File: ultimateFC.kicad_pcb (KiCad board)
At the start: 6 copper layers, 36 x 36 mm, 213 parts, among them J1 USB_B_Micro, SW1 SW_Push, U1 LMR33630CQRNX, U2 TPS62824ADMQ, U3 LMR33620CRNXT, U4 S25FL064L, U5 DPS310, U6 BMI270, U7 STM32H735VGH6, U8 ICM-20602, Y1 CSTNE8M00G550000R0

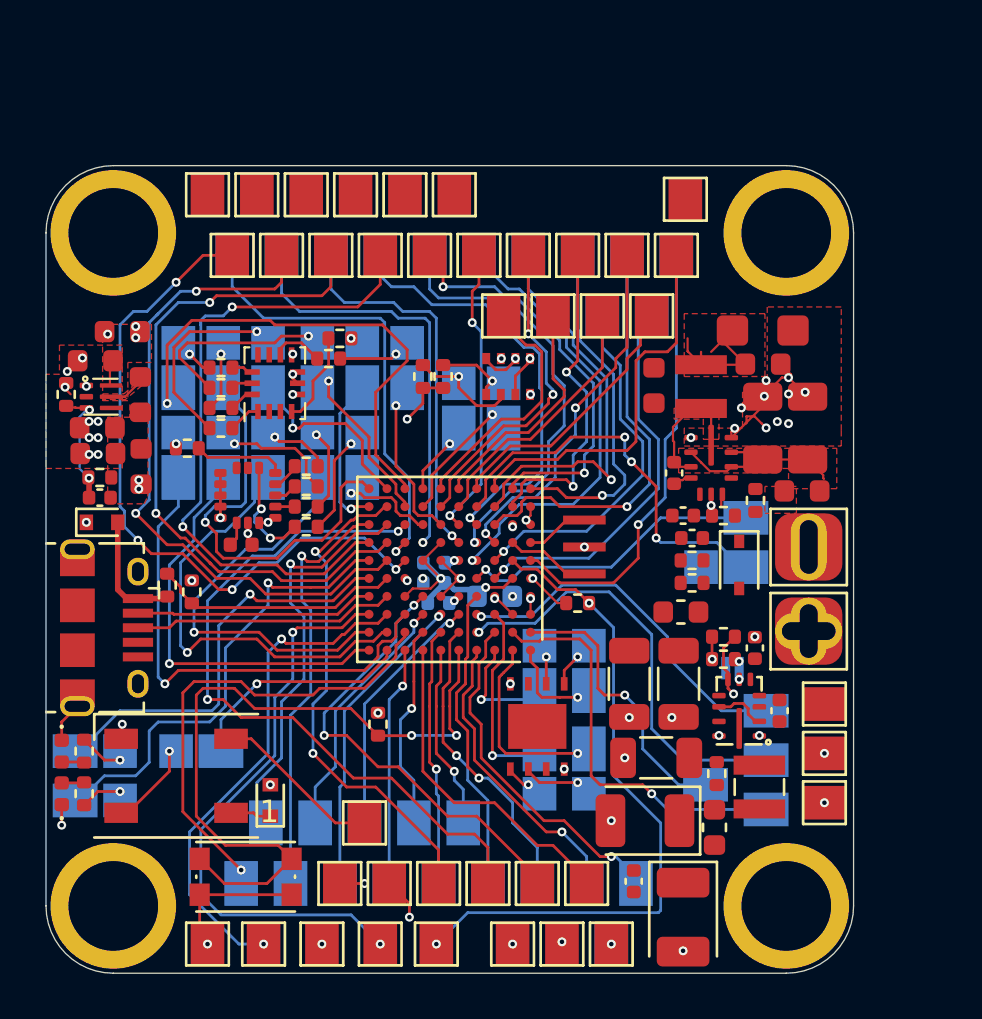
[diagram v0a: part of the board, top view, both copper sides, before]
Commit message: MORE PADS!!!
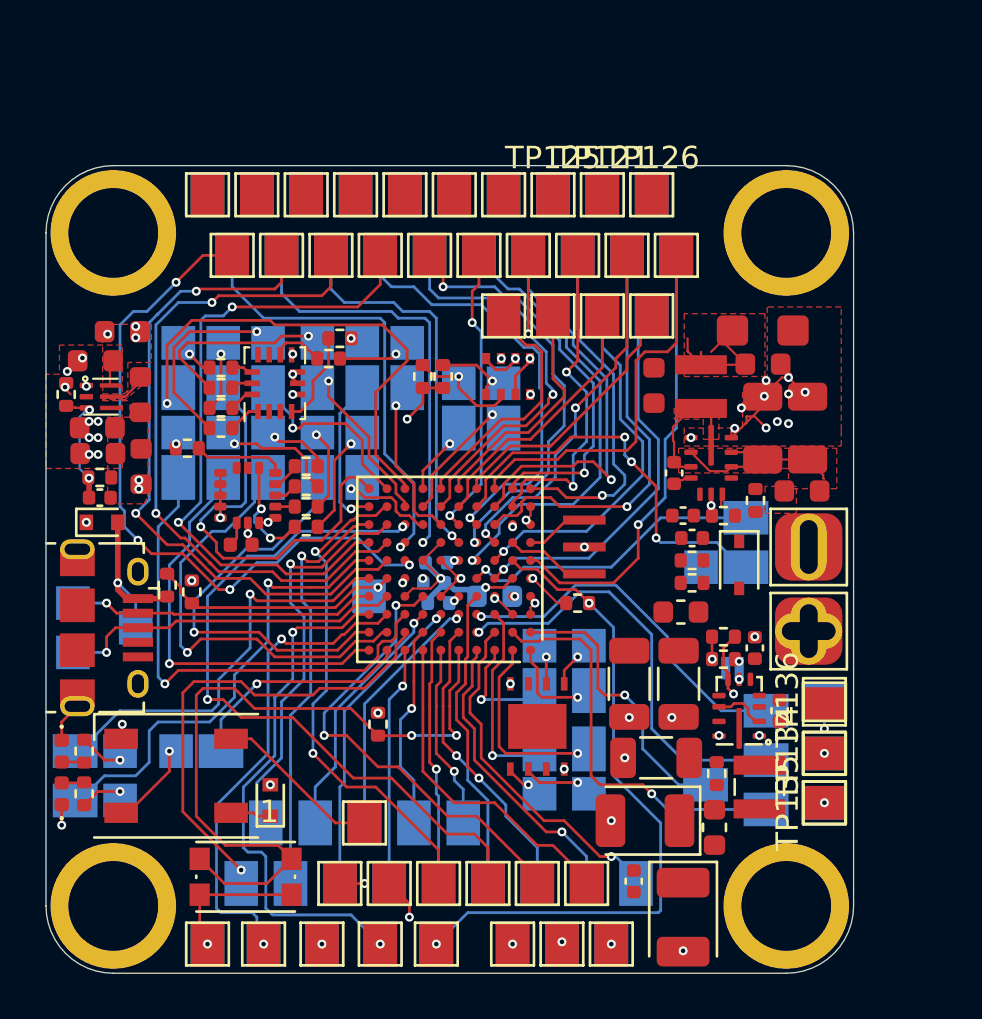
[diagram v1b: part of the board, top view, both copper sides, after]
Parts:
- added TP117: Pad, TestPoint:TestPoint_Pad_1.5x1.5mm, B.Cu at (111.4, 116.2)
- added TP118: Pad, TestPoint:TestPoint_Pad_1.5x1.5mm, B.Cu at (101.0, 117.6)
- added TP119: Pad, TestPoint:TestPoint_Pad_1.5x1.5mm, B.Cu at (98.2, 116.5)
- added TP120: Pad, TestPoint:TestPoint_Pad_1.5x1.5mm, B.Cu at (98.2, 118.7)
- added TP121: Pad, TestPoint:TestPoint_Pad_1.5x1.5mm, F.Cu at (121.8, 98.3)
- added TP122: Pad, TestPoint:TestPoint_Pad_1.5x1.5mm, B.Cu at (121.8, 98.3)
- added TP123: Pad, TestPoint:TestPoint_Pad_1.5x1.5mm, B.Cu at (108.6, 98.3)
- added TP124: Pad, TestPoint:TestPoint_Pad_1.5x1.5mm, B.Cu at (106.4, 98.3)
- added TP125: Pad, TestPoint:TestPoint_Pad_1.5x1.5mm, F.Cu at (119.6, 98.3)
- added TP126: Pad, TestPoint:TestPoint_Pad_1.5x1.5mm, F.Cu at (124.0, 98.3)
- added TP127: Pad, TestPoint:TestPoint_Pad_1.5x1.5mm, B.Cu at (110.8, 98.3)
- added TP128: Pad, TestPoint:TestPoint_Pad_1.5x1.5mm, B.Cu at (119.6, 98.3)
- added TP129: Pad, TestPoint:TestPoint_Pad_1.5x1.5mm, B.Cu at (117.4, 98.3)
- added TP130: Pad, TestPoint:TestPoint_Pad_1.5x1.5mm, B.Cu at (124.0, 98.3)
- added TP131: Pad, TestPoint:TestPoint_Pad_1.5x1.5mm, B.Cu at (115.2, 98.3)
- added TP132: Pad, TestPoint:TestPoint_Pad_1.5x1.5mm, B.Cu at (113.0, 98.3)
- added TP133: Pad, TestPoint:TestPoint_Pad_1.5x1.5mm, B.Cu at (104.2, 98.3)
- added TP134: Pad, TestPoint:TestPoint_Pad_1.5x1.5mm, F.Cu at (131.7, 123.2)
- added TP135: Pad, TestPoint:TestPoint_Pad_1.5x1.5mm, F.Cu at (131.7, 125.4)
- added TP136: Pad, TestPoint:TestPoint_Pad_1.5x1.5mm, F.Cu at (131.7, 120.8)
- added TP137: Pad, TestPoint:TestPoint_Pad_1.5x1.5mm, B.Cu at (111.9, 131.7)
- added TP138: Pad, TestPoint:TestPoint_Pad_1.5x1.5mm, B.Cu at (106.7, 131.7)
- added TP139: Pad, TestPoint:TestPoint_Pad_1.5x1.5mm, B.Cu at (114.4, 131.7)
- added TP140: Pad, TestPoint:TestPoint_Pad_1.5x1.5mm, B.Cu at (109.3, 131.7)
- added TP141: Pad, TestPoint:TestPoint_Pad_1.5x1.5mm, B.Cu at (104.2, 131.7)
- added TP142: Pad, TestPoint:TestPoint_Pad_1.5x1.5mm, B.Cu at (117.8, 131.7)
- added TP143: Pad, TestPoint:TestPoint_Pad_1.5x1.5mm, B.Cu at (120.0, 131.7)
- moved TP5 10.3 mm to (115.2, 98.3)
- moved TP4 8.80 mm to (117.4, 98.3)
- moved TP2 6.60 mm to (113.0, 98.3)
- moved TP7 6.60 mm to (106.4, 98.3)
- moved TP8 4.40 mm to (110.8, 98.3)
- moved TP3 2.20 mm to (108.6, 98.3)
- moved C38 0.10 mm to (114.4, 114.7)
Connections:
- net /SWDCLK renamed SWDCLK
- net /SWDIO renamed SWDIO
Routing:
- net Net-(J1-Pad3): track 11.7 -> 15.4 mm, vias 0 -> 1
- net Net-(J1-Pad2): track 10.7 -> 13.7 mm, vias 0 -> 1
- net SWDIO: track 26.0 -> 23.5 mm
- net USB_VBUS: track 5.40 -> 7.73 mm, vias 0 -> 1
- net +3V3: track 18.7 -> 20.1 mm, vias 15 -> 16
- net SWDCLK: track 22.6 -> 21.8 mm
- net /USB_VBUS_sense: vias 0 -> 1
